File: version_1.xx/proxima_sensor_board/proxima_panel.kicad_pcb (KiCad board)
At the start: 2 copper layers, 83 x 94 mm, 587 parts, among them J1 Conn_01x03, U1 TSOP32156, U2 NE555D

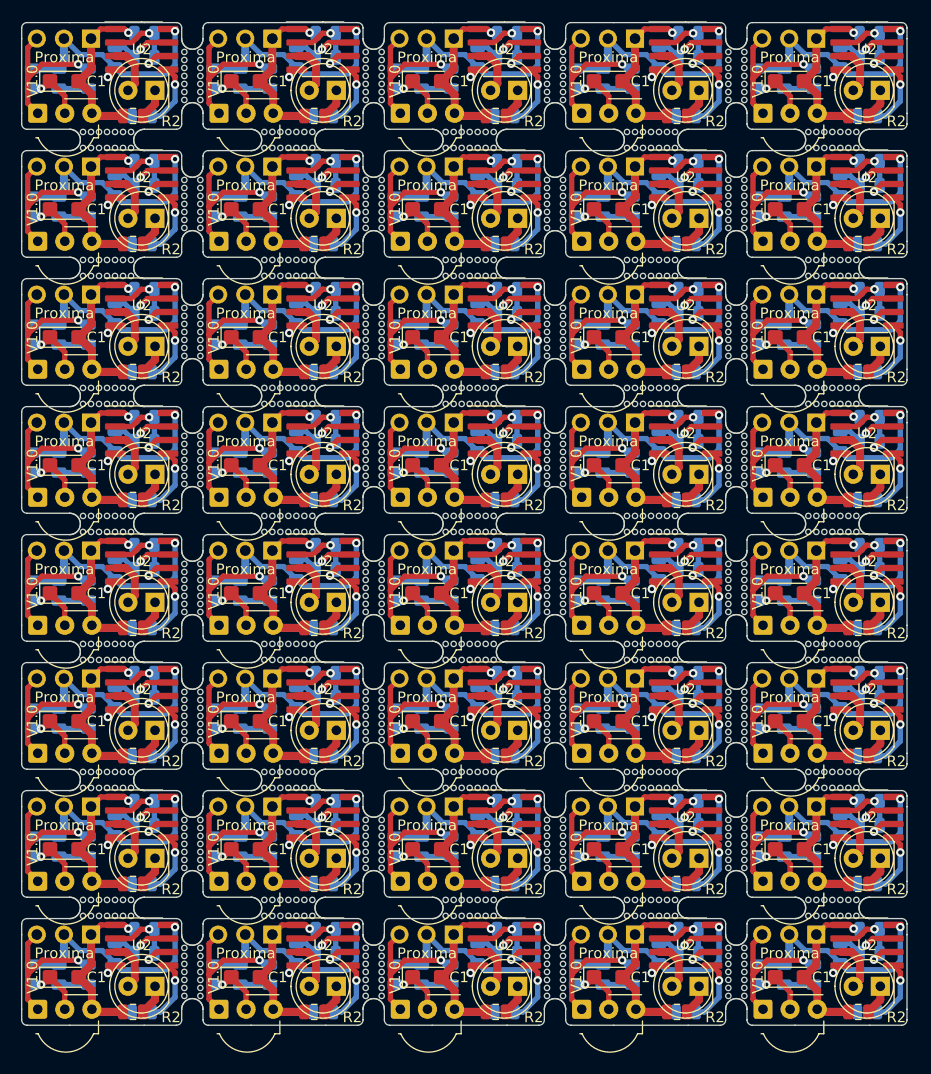
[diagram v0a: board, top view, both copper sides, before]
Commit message: panelization 2
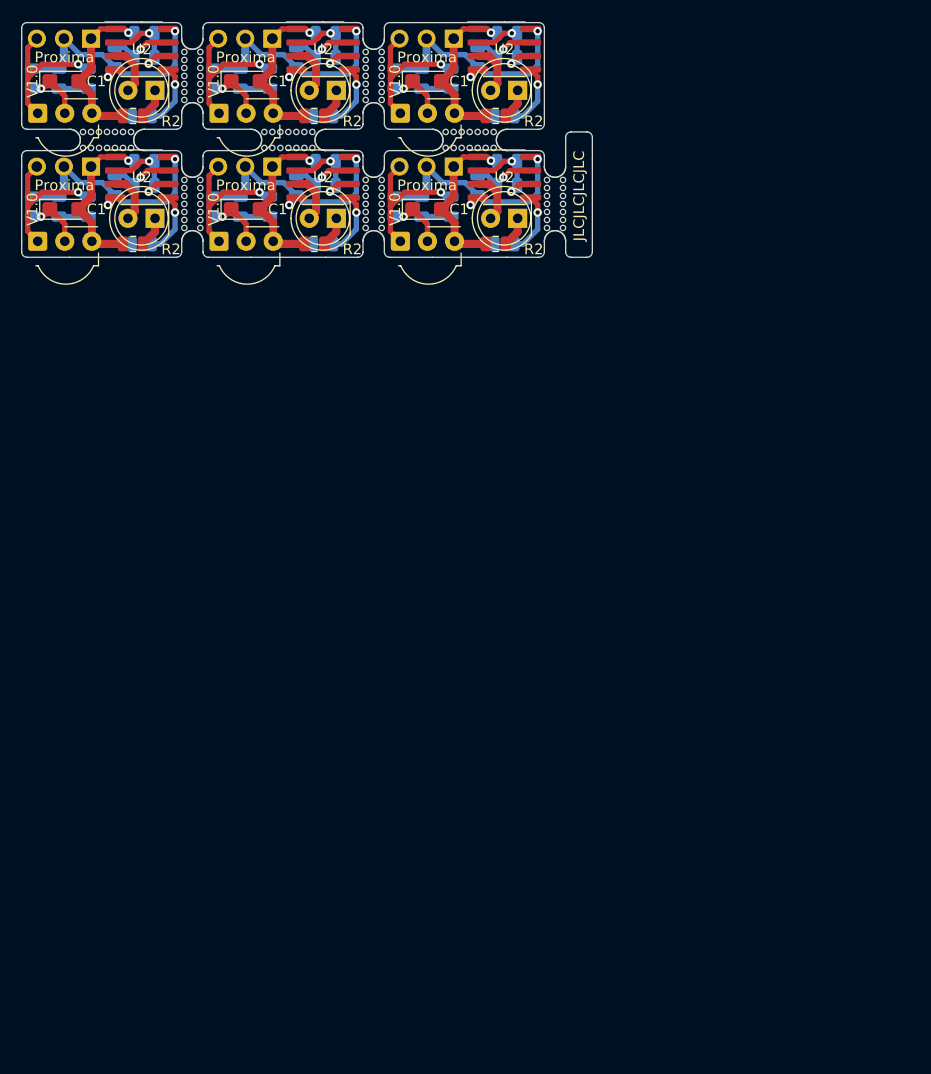
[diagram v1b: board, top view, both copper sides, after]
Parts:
- removed the ? at (199.0, 162.0)
- removed the ? at (182.0, 162.0)
- removed the ? at (165.0, 162.0)
- removed the ? at (148.0, 162.0)
- removed the ? at (199.0, 150.0)
- removed the ? at (182.0, 150.0)
- removed the ? at (165.0, 150.0)
- removed the ? at (148.0, 150.0)
- removed the ? at (199.0, 138.0)
- removed the ? at (182.0, 138.0)
- removed the ? at (199.0, 186.0)
- removed the ? at (165.0, 138.0)
- removed the ? at (148.0, 138.0)
- removed the ? at (199.0, 126.0)
- removed the ? at (182.0, 126.0)
- removed the ? at (165.0, 126.0)
- removed the ? at (148.0, 126.0)
- removed the ? at (199.0, 114.0)
- removed the ? at (182.0, 186.0)
- removed the ? at (199.0, 102.0)
- removed the ? at (182.0, 102.0)
- removed the ? at (208.0, 180.0)
- removed the ? at (191.0, 180.0)
- removed the ? at (174.0, 180.0)
- removed the ? at (157.0, 180.0)
- removed the ? at (140.0, 180.0)
- removed the ? at (208.0, 168.0)
- removed the ? at (191.0, 168.0)
- removed the ? at (174.0, 168.0)
- removed the ? at (165.0, 186.0)
- removed the ? at (157.0, 168.0)
- removed the ? at (140.0, 168.0)
- removed the ? at (208.0, 156.0)
- removed the ? at (191.0, 156.0)
- removed the ? at (174.0, 156.0)
- removed the ? at (157.0, 156.0)
- removed the ? at (140.0, 156.0)
- removed the ? at (208.0, 144.0)
- removed the ? at (191.0, 144.0)
- removed the ? at (174.0, 144.0)
- removed the ? at (148.0, 186.0)
- removed the ? at (157.0, 144.0)
- removed the ? at (140.0, 144.0)
- removed the ? at (208.0, 132.0)
- removed the ? at (191.0, 132.0)
- removed the ? at (174.0, 132.0)
- removed the ? at (157.0, 132.0)
- removed the ? at (140.0, 132.0)
- removed the ? at (208.0, 120.0)
- removed the ? at (191.0, 120.0)
- removed the ? at (174.0, 120.0)
- removed the ? at (199.0, 174.0)
- removed the ? at (157.0, 120.0)
- removed the ? at (140.0, 120.0)
- removed the ? at (208.0, 108.0)
- removed the ? at (191.0, 108.0)
- removed the ? at (182.0, 174.0)
- removed the ? at (165.0, 174.0)
- removed the ? at (148.0, 174.0)
- removed the C1 at (204.0, 186.5)
- removed the C1 at (136.0, 174.5)
- removed the C1 at (204.0, 162.5)
- removed the C1 at (187.0, 162.5)
- removed the C1 at (170.0, 162.5)
- removed the C1 at (153.0, 162.5)
- removed the C1 at (136.0, 162.5)
- removed the C1 at (204.0, 150.5)
- removed the C1 at (187.0, 150.5)
- removed the C1 at (170.0, 150.5)
- removed the C1 at (153.0, 150.5)
- removed the C1 at (187.0, 186.5)
- removed the C1 at (136.0, 150.5)
- removed the C1 at (204.0, 138.5)
- removed the C1 at (187.0, 138.5)
- removed the C1 at (170.0, 138.5)
- removed the C1 at (153.0, 138.5)
- removed the C1 at (136.0, 138.5)
- removed the C1 at (204.0, 126.5)
- removed the C1 at (187.0, 126.5)
- removed the C1 at (170.0, 126.5)
- removed the C1 at (153.0, 126.5)
- removed the C1 at (170.0, 186.5)
- removed the C1 at (136.0, 126.5)
- removed the C1 at (204.0, 114.5)
- removed the C1 at (187.0, 114.5)
- removed the C1 at (204.0, 102.5)
- removed the C1 at (187.0, 102.5)
- removed the C1 at (153.0, 186.5)
- removed the C1 at (136.0, 186.5)
- removed the C1 at (204.0, 174.5)
- removed the C1 at (187.0, 174.5)
- removed the C1 at (170.0, 174.5)
- removed the C1 at (153.0, 174.5)
- removed the C2 at (211.2, 189.8)
- removed the C2 at (143.2, 177.8)
- removed the C2 at (211.2, 165.8)
- removed the C2 at (194.2, 165.8)
- removed the C2 at (177.2, 165.8)
- removed the C2 at (160.2, 165.8)
- removed the C2 at (143.2, 165.8)
- removed the C2 at (211.2, 153.8)
- removed the C2 at (194.2, 153.8)
- removed the C2 at (177.2, 153.8)
- removed the C2 at (160.2, 153.8)
- removed the C2 at (194.2, 189.8)
- removed the C2 at (143.2, 153.8)
- removed the C2 at (211.2, 141.8)
- removed the C2 at (194.2, 141.8)
- removed the C2 at (177.2, 141.8)
- removed the C2 at (160.2, 141.8)
- removed the C2 at (143.2, 141.8)
- removed the C2 at (211.2, 129.8)
- removed the C2 at (194.2, 129.8)
- removed the C2 at (177.2, 129.8)
- removed the C2 at (160.2, 129.8)
- removed the C2 at (177.2, 189.8)
- removed the C2 at (143.2, 129.8)
- removed the C2 at (211.2, 117.8)
- removed the C2 at (194.2, 117.8)
- removed the C2 at (211.2, 105.8)
- removed the C2 at (194.2, 105.8)
- removed the C2 at (160.2, 189.8)
- removed the C2 at (143.2, 189.8)
- removed the C2 at (211.2, 177.8)
- removed the C2 at (194.2, 177.8)
- removed the C2 at (177.2, 177.8)
- removed the C2 at (160.2, 177.8)
- removed the C3 at (211.5, 182.0)
- removed the C3 at (143.5, 170.0)
- removed the C3 at (211.5, 158.0)
- removed the C3 at (194.5, 158.0)
- removed the C3 at (177.5, 158.0)
- removed the C3 at (160.5, 158.0)
- removed the C3 at (143.5, 158.0)
- removed the C3 at (211.5, 146.0)
- removed the C3 at (194.5, 146.0)
- removed the C3 at (177.5, 146.0)
- removed the C3 at (160.5, 146.0)
- removed the C3 at (194.5, 182.0)
- removed the C3 at (143.5, 146.0)
- removed the C3 at (211.5, 134.0)
- removed the C3 at (194.5, 134.0)
- removed the C3 at (177.5, 134.0)
- removed the C3 at (160.5, 134.0)
- removed the C3 at (143.5, 134.0)
- removed the C3 at (211.5, 122.0)
- removed the C3 at (194.5, 122.0)
- removed the C3 at (177.5, 122.0)
- removed the C3 at (160.5, 122.0)
- removed the C3 at (177.5, 182.0)
- removed the C3 at (143.5, 122.0)
- removed the C3 at (211.5, 110.0)
- removed the C3 at (194.5, 110.0)
- removed the C3 at (211.5, 98.0)
- removed the C3 at (194.5, 98.0)
- removed the C3 at (160.5, 182.0)
- removed the C3 at (143.5, 182.0)
- removed the C3 at (211.5, 170.0)
- removed the C3 at (194.5, 170.0)
- removed the C3 at (177.5, 170.0)
- removed the C3 at (160.5, 170.0)
- removed the D1 at (212.5, 187.3)
- removed the D1 at (144.5, 175.3)
- removed the D1 at (212.5, 163.3)
- removed the D1 at (195.5, 163.3)
- removed the D1 at (178.5, 163.3)
- removed the D1 at (161.5, 163.3)
- removed the D1 at (144.5, 163.3)
- removed the D1 at (212.5, 151.3)
- removed the D1 at (195.5, 151.3)
- removed the D1 at (178.5, 151.3)
- removed the D1 at (161.5, 151.3)
- removed the D1 at (195.5, 187.3)
- removed the D1 at (144.5, 151.3)
- removed the D1 at (212.5, 139.3)
- removed the D1 at (195.5, 139.3)
- removed the D1 at (178.5, 139.3)
- removed the D1 at (161.5, 139.3)
- removed the D1 at (144.5, 139.3)
- removed the D1 at (212.5, 127.3)
- removed the D1 at (195.5, 127.3)
- removed the D1 at (178.5, 127.3)
- removed the D1 at (161.5, 127.3)
- removed the D1 at (178.5, 187.3)
- removed the D1 at (144.5, 127.3)
- removed the D1 at (212.5, 115.3)
- removed the D1 at (195.5, 115.3)
- removed the D1 at (212.5, 103.3)
- removed the D1 at (195.5, 103.3)
- removed the D1 at (161.5, 187.3)
- removed the D1 at (144.5, 187.3)
- removed the D1 at (212.5, 175.3)
- removed the D1 at (195.5, 175.3)
- removed the D1 at (178.5, 175.3)
- removed the D1 at (161.5, 175.3)
- removed the D2 at (203.5, 186.2)
- removed the D2 at (135.5, 174.2)
- removed the D2 at (203.5, 162.2)
- removed the D2 at (186.5, 162.2)
- removed the D2 at (169.5, 162.2)
- removed the D2 at (152.5, 162.2)
- removed the D2 at (135.5, 162.2)
- removed the D2 at (203.5, 150.2)
- removed the D2 at (186.5, 150.2)
- removed the D2 at (169.5, 150.2)
- removed the D2 at (152.5, 150.2)
- removed the D2 at (186.5, 186.2)
- removed the D2 at (135.5, 150.2)
- removed the D2 at (203.5, 138.2)
- removed the D2 at (186.5, 138.2)
- removed the D2 at (169.5, 138.2)
- removed the D2 at (152.5, 138.2)
- removed the D2 at (135.5, 138.2)
- removed the D2 at (203.5, 126.2)
- removed the D2 at (186.5, 126.2)
- removed the D2 at (169.5, 126.2)
- removed the D2 at (152.5, 126.2)
- removed the D2 at (169.5, 186.2)
- removed the D2 at (135.5, 126.2)
- removed the D2 at (203.5, 114.2)
- removed the D2 at (186.5, 114.2)
- removed the D2 at (203.5, 102.2)
- removed the D2 at (186.5, 102.2)
- removed the D2 at (152.5, 186.2)
- removed the D2 at (135.5, 186.2)
- removed the D2 at (203.5, 174.2)
- removed the D2 at (186.5, 174.2)
- removed the D2 at (169.5, 174.2)
- removed the D2 at (152.5, 174.2)
- removed the J1 at (206.5, 182.5)
- removed the J1 at (138.5, 170.5)
- removed the J1 at (206.5, 158.5)
- removed the J1 at (189.5, 158.5)
- removed the J1 at (172.5, 158.5)
- removed the J1 at (155.5, 158.5)
- removed the J1 at (138.5, 158.5)
- removed the J1 at (206.5, 146.5)
- removed the J1 at (189.5, 146.5)
- removed the J1 at (172.5, 146.5)
- removed the J1 at (155.5, 146.5)
- removed the J1 at (189.5, 182.5)
- removed the J1 at (138.5, 146.5)
- removed the J1 at (206.5, 134.5)
- removed the J1 at (189.5, 134.5)
- removed the J1 at (172.5, 134.5)
- removed the J1 at (155.5, 134.5)
- removed the J1 at (138.5, 134.5)
- removed the J1 at (206.5, 122.5)
- removed the J1 at (189.5, 122.5)
- removed the J1 at (172.5, 122.5)
- removed the J1 at (155.5, 122.5)
- removed the J1 at (172.5, 182.5)
- removed the J1 at (138.5, 122.5)
- removed the J1 at (206.5, 110.5)
- removed the J1 at (189.5, 110.5)
- removed the J1 at (206.5, 98.5)
- removed the J1 at (189.5, 98.5)
- removed the J1 at (155.5, 182.5)
- removed the J1 at (138.5, 182.5)
- removed the J1 at (206.5, 170.5)
- removed the J1 at (189.5, 170.5)
- removed the J1 at (172.5, 170.5)
- removed the J1 at (155.5, 170.5)
- removed the R1 at (201.0, 186.2)
- removed the R1 at (133.0, 174.2)
- removed the R1 at (201.0, 162.2)
- removed the R1 at (184.0, 162.2)
- removed the R1 at (167.0, 162.2)
- removed the R1 at (150.0, 162.2)
- removed the R1 at (133.0, 162.2)
- removed the R1 at (201.0, 150.2)
- removed the R1 at (184.0, 150.2)
- removed the R1 at (167.0, 150.2)
- removed the R1 at (150.0, 150.2)
- removed the R1 at (184.0, 186.2)
- removed the R1 at (133.0, 150.2)
- removed the R1 at (201.0, 138.2)
- removed the R1 at (184.0, 138.2)
- removed the R1 at (167.0, 138.2)
- removed the R1 at (150.0, 138.2)
- removed the R1 at (133.0, 138.2)
- removed the R1 at (201.0, 126.2)
- removed the R1 at (184.0, 126.2)
- removed the R1 at (167.0, 126.2)
- removed the R1 at (150.0, 126.2)
- removed the R1 at (167.0, 186.2)
- removed the R1 at (133.0, 126.2)
- removed the R1 at (201.0, 114.2)
- removed the R1 at (184.0, 114.2)
- removed the R1 at (201.0, 102.2)
- removed the R1 at (184.0, 102.2)
- removed the R1 at (150.0, 186.2)
- removed the R1 at (133.0, 186.2)
- removed the R1 at (201.0, 174.2)
- removed the R1 at (184.0, 174.2)
- removed the R1 at (167.0, 174.2)
- removed the R1 at (150.0, 174.2)
- removed the R2 at (210.4, 189.8)
- removed the R2 at (142.4, 177.8)
- removed the R2 at (210.4, 165.8)
- removed the R2 at (193.4, 165.8)
- removed the R2 at (176.4, 165.8)
- removed the R2 at (159.4, 165.8)
- removed the R2 at (142.4, 165.8)
- removed the R2 at (210.4, 153.8)
- removed the R2 at (193.4, 153.8)
- removed the R2 at (176.4, 153.8)
- removed the R2 at (159.4, 153.8)
- removed the R2 at (193.4, 189.8)
- removed the R2 at (142.4, 153.8)
- removed the R2 at (210.4, 141.8)
- removed the R2 at (193.4, 141.8)
- removed the R2 at (176.4, 141.8)
- removed the R2 at (159.4, 141.8)
- removed the R2 at (142.4, 141.8)
- removed the R2 at (210.4, 129.8)
- removed the R2 at (193.4, 129.8)
- removed the R2 at (176.4, 129.8)
- removed the R2 at (159.4, 129.8)
- removed the R2 at (176.4, 189.8)
- removed the R2 at (142.4, 129.8)
- removed the R2 at (210.4, 117.8)
- removed the R2 at (193.4, 117.8)
- removed the R2 at (210.4, 105.8)
- removed the R2 at (193.4, 105.8)
- removed the R2 at (159.4, 189.8)
- removed the R2 at (142.4, 189.8)
- removed the R2 at (210.4, 177.8)
- removed the R2 at (193.4, 177.8)
- removed the R2 at (176.4, 177.8)
- removed the R2 at (159.4, 177.8)
- removed the R3 at (208.8, 184.2)
- removed the R3 at (140.8, 172.2)
- removed the R3 at (208.8, 160.2)
- removed the R3 at (191.8, 160.2)
- removed the R3 at (174.8, 160.2)
- removed the R3 at (157.8, 160.2)
- removed the R3 at (140.8, 160.2)
- removed the R3 at (208.8, 148.2)
- removed the R3 at (191.8, 148.2)
- removed the R3 at (174.8, 148.2)
- removed the R3 at (157.8, 148.2)
- removed the R3 at (191.8, 184.2)
- removed the R3 at (140.8, 148.2)
- removed the R3 at (208.8, 136.2)
- removed the R3 at (191.8, 136.2)
- removed the R3 at (174.8, 136.2)
- removed the R3 at (157.8, 136.2)
- removed the R3 at (140.8, 136.2)
- removed the R3 at (208.8, 124.2)
- removed the R3 at (191.8, 124.2)
- removed the R3 at (174.8, 124.2)
- removed the R3 at (157.8, 124.2)
- removed the R3 at (174.8, 184.2)
- removed the R3 at (140.8, 124.2)
- removed the R3 at (208.8, 112.2)
- removed the R3 at (191.8, 112.2)
- removed the R3 at (208.8, 100.2)
- removed the R3 at (191.8, 100.2)
- removed the R3 at (157.8, 184.2)
- removed the R3 at (140.8, 184.2)
- removed the R3 at (208.8, 172.2)
- removed the R3 at (191.8, 172.2)
- removed the R3 at (174.8, 172.2)
- removed the R3 at (157.8, 172.2)
- removed the R4 at (211.5, 184.2)
- removed the R4 at (143.5, 172.2)
- removed the R4 at (211.5, 160.2)
- removed the R4 at (194.5, 160.2)
- removed the R4 at (177.5, 160.2)
- removed the R4 at (160.5, 160.2)
- removed the R4 at (143.5, 160.2)
- removed the R4 at (211.5, 148.2)
- removed the R4 at (194.5, 148.2)
- removed the R4 at (177.5, 148.2)
- removed the R4 at (160.5, 148.2)
- removed the R4 at (194.5, 184.2)
- removed the R4 at (143.5, 148.2)
- removed the R4 at (211.5, 136.2)
- removed the R4 at (194.5, 136.2)
- removed the R4 at (177.5, 136.2)
- removed the R4 at (160.5, 136.2)
- removed the R4 at (143.5, 136.2)
- removed the R4 at (211.5, 124.2)
- removed the R4 at (194.5, 124.2)
- removed the R4 at (177.5, 124.2)
- removed the R4 at (160.5, 124.2)
- removed the R4 at (177.5, 184.2)
- removed the R4 at (143.5, 124.2)
- removed the R4 at (211.5, 112.2)
- removed the R4 at (194.5, 112.2)
- removed the R4 at (211.5, 100.2)
- removed the R4 at (194.5, 100.2)
- removed the R4 at (160.5, 184.2)
- removed the R4 at (143.5, 184.2)
- removed the R4 at (211.5, 172.2)
- removed the R4 at (194.5, 172.2)
- removed the R4 at (177.5, 172.2)
- removed the R4 at (160.5, 172.2)
- removed the R5 at (206.2, 186.2)
- removed the R5 at (138.2, 174.2)
- removed the R5 at (206.2, 162.2)
- removed the R5 at (189.2, 162.2)
- removed the R5 at (172.2, 162.2)
- removed the R5 at (155.2, 162.2)
- removed the R5 at (138.2, 162.2)
- removed the R5 at (206.2, 150.2)
- removed the R5 at (189.2, 150.2)
- removed the R5 at (172.2, 150.2)
- removed the R5 at (155.2, 150.2)
- removed the R5 at (189.2, 186.2)
- removed the R5 at (138.2, 150.2)
- removed the R5 at (206.2, 138.2)
- removed the R5 at (189.2, 138.2)
- removed the R5 at (172.2, 138.2)
- removed the R5 at (155.2, 138.2)
- removed the R5 at (138.2, 138.2)
- removed the R5 at (206.2, 126.2)
- removed the R5 at (189.2, 126.2)
- removed the R5 at (172.2, 126.2)
- removed the R5 at (155.2, 126.2)
- removed the R5 at (172.2, 186.2)
- removed the R5 at (138.2, 126.2)
- removed the R5 at (206.2, 114.2)
- removed the R5 at (189.2, 114.2)
- removed the R5 at (206.2, 102.2)
- removed the R5 at (189.2, 102.2)
- removed the R5 at (155.2, 186.2)
- removed the R5 at (138.2, 186.2)
- removed the R5 at (206.2, 174.2)
- removed the R5 at (189.2, 174.2)
- removed the R5 at (172.2, 174.2)
- removed the R5 at (155.2, 174.2)
- removed the U1 at (201.5, 189.5)
- removed the U1 at (133.5, 177.5)
- removed the U1 at (201.5, 165.5)
- removed the U1 at (184.5, 165.5)
- removed the U1 at (167.5, 165.5)
- removed the U1 at (150.5, 165.5)
- removed the U1 at (133.5, 165.5)
- removed the U1 at (201.5, 153.5)
- removed the U1 at (184.5, 153.5)
- removed the U1 at (167.5, 153.5)
- removed the U1 at (150.5, 153.5)
- removed the U1 at (184.5, 189.5)
- removed the U1 at (133.5, 153.5)
- removed the U1 at (201.5, 141.5)
- removed the U1 at (184.5, 141.5)
- removed the U1 at (167.5, 141.5)
- removed the U1 at (150.5, 141.5)
- removed the U1 at (133.5, 141.5)
- removed the U1 at (201.5, 129.5)
- removed the U1 at (184.5, 129.5)
- removed the U1 at (167.5, 129.5)
- removed the U1 at (150.5, 129.5)
- removed the U1 at (167.5, 189.5)
- removed the U1 at (133.5, 129.5)
- removed the U1 at (201.5, 117.5)
- removed the U1 at (184.5, 117.5)
- removed the U1 at (201.5, 105.5)
- removed the U1 at (184.5, 105.5)
- removed the U1 at (150.5, 189.5)
- removed the U1 at (133.5, 189.5)
- removed the U1 at (201.5, 177.5)
- removed the U1 at (184.5, 177.5)
- removed the U1 at (167.5, 177.5)
- removed the U1 at (150.5, 177.5)
- removed the U2 at (211.2, 183.5)
- removed the U2 at (143.2, 171.5)
- removed the U2 at (211.2, 159.5)
- removed the U2 at (194.2, 159.5)
- removed the U2 at (177.2, 159.5)
- removed the U2 at (160.2, 159.5)
- removed the U2 at (143.2, 159.5)
- removed the U2 at (211.2, 147.5)
- removed the U2 at (194.2, 147.5)
- removed the U2 at (177.2, 147.5)
- removed the U2 at (160.2, 147.5)
- removed the U2 at (194.2, 183.5)
- removed the U2 at (143.2, 147.5)
- removed the U2 at (211.2, 135.5)
- removed the U2 at (194.2, 135.5)
- removed the U2 at (177.2, 135.5)
- removed the U2 at (160.2, 135.5)
- removed the U2 at (143.2, 135.5)
- removed the U2 at (211.2, 123.5)
- removed the U2 at (194.2, 123.5)
- removed the U2 at (177.2, 123.5)
- removed the U2 at (160.2, 123.5)
- removed the U2 at (177.2, 183.5)
- removed the U2 at (143.2, 123.5)
- removed the U2 at (211.2, 111.5)
- removed the U2 at (194.2, 111.5)
- removed the U2 at (211.2, 99.5)
- removed the U2 at (194.2, 99.5)
- removed the U2 at (160.2, 183.5)
- removed the U2 at (143.2, 183.5)
- removed the U2 at (211.2, 171.5)
- removed the U2 at (194.2, 171.5)
- removed the U2 at (177.2, 171.5)
- removed the U2 at (160.2, 171.5)
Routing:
- net VCC: track 948.4 -> 142.3 mm, vias 80 -> 12
- net GND: track 778.0 -> 116.7 mm, vias 40 -> 6
- net OUTPUT_INVERTED: track 565.6 -> 84.8 mm, vias 40 -> 6
- net Net-(C3-Pad1): track 397.0 -> 59.5 mm, vias 80 -> 12
- net Net-(R3-Pad2): track 241.3 -> 36.2 mm, vias 40 -> 6
- net Net-(C2-Pad1): track 239.9 -> 36.0 mm, vias 40 -> 6
- net Net-(C1-Pad1): track 220.8 -> 33.1 mm, vias 40 -> 6
- net SQUARE_WAVE_SIGNAL: track 193.1 -> 29.0 mm
- net Net-(D1-Pad1): track 114.6 -> 17.2 mm
- net Net-(D2-Pad1): track 110.0 -> 16.5 mm
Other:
- board size 83 x 94 mm -> 53.5 x 22 mm
- board text added: "JLCJLCJLCJLC"
